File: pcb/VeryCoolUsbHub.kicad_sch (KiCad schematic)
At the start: 58 parts, among them U1 HD3SS3220RNHR, U2 HD3SS3220RNHR, X1 X322525MSB4SI, X2 X322525MSB4SI

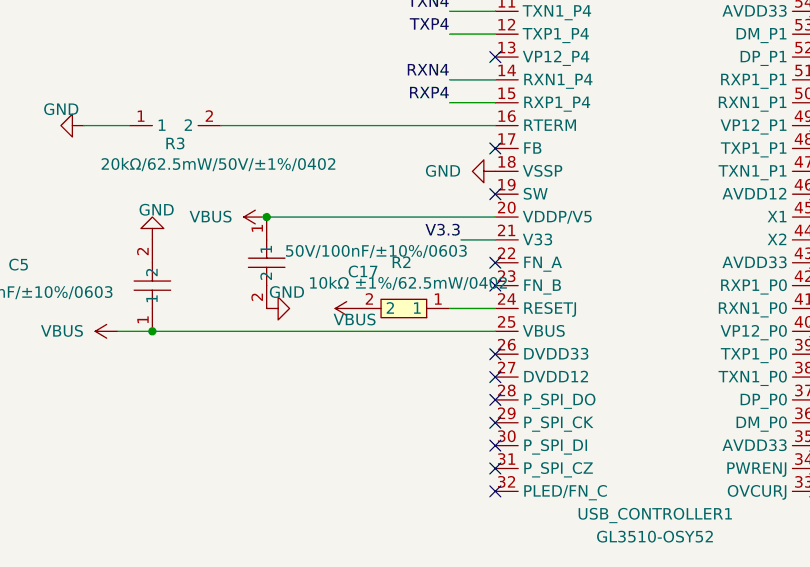
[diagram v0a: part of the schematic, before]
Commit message: maybedone?
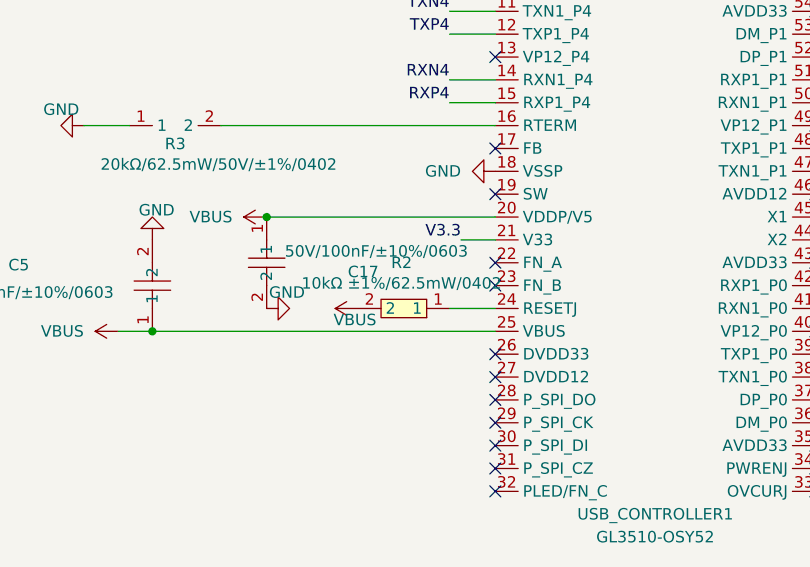
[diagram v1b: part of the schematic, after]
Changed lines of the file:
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@@
 		)
 		(property "Description" "10kΩ ±1%/62.5mW/0402"
-			(at 99.568 255.016 0)
+			(at 98.806 255.016 0)
 			(effects
 				(font
@@
 			)
 		)
-		(property "Datasheet" "https://www.lcsc.com/datasheet/C871499.pdf"
+		(property "Datasheet" "https://www.lcsc.com/datasheet/C871726.pdf"
 			(at 193.04 93.98 0)
 			(effects
